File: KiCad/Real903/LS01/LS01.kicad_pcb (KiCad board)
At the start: 2 copper layers, 50.8 x 19 mm, 24 parts, among them J1 Conn_01x06, J2 Conn_01x03, J3 Conn_01x03

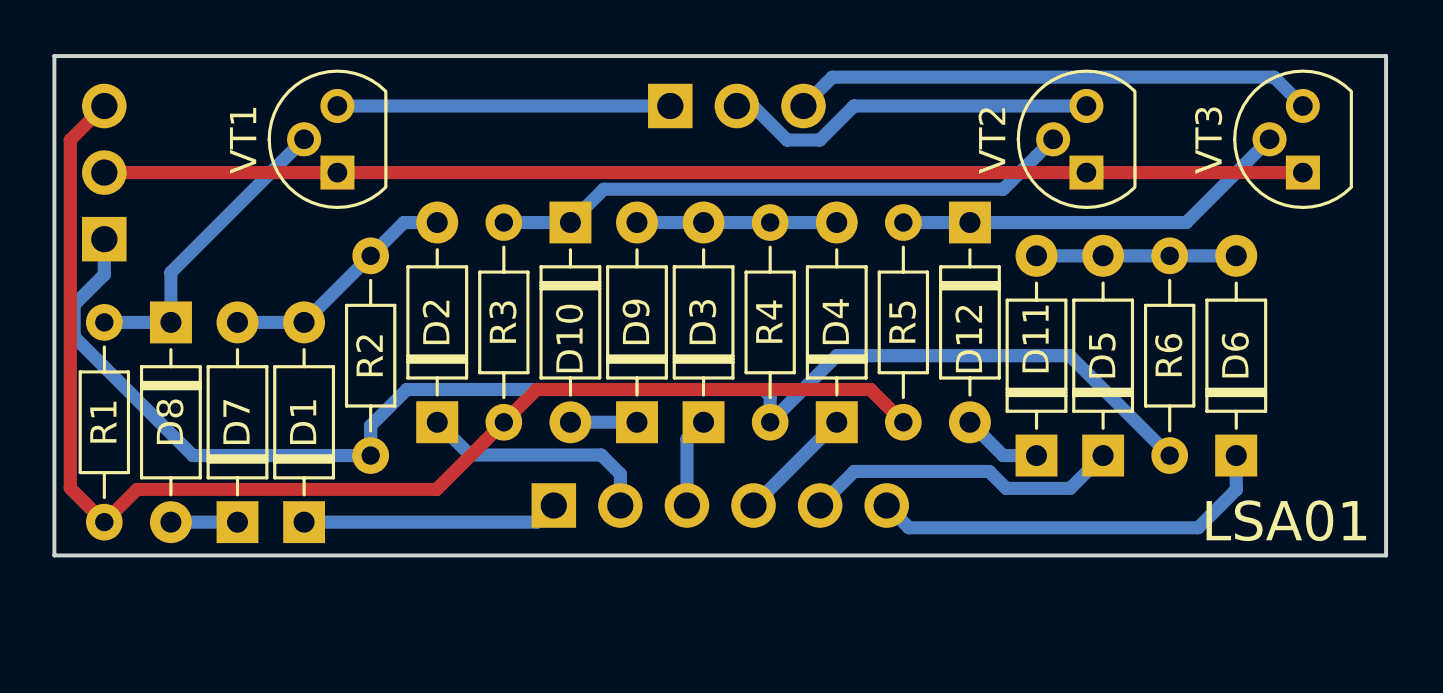
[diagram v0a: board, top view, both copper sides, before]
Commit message: New Kicad design files
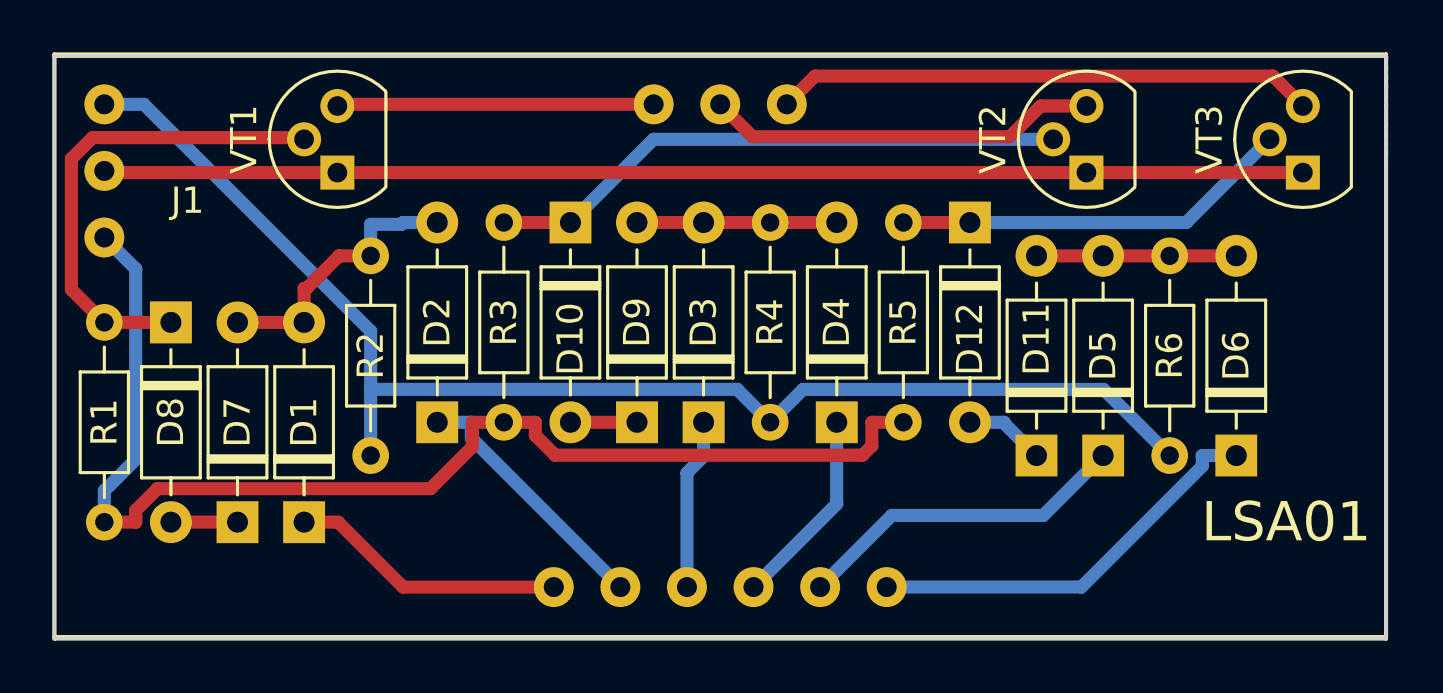
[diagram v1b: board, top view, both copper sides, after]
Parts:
- removed J2, J3: Conn_01x03, ELLIOTT:PinHeader_1x03_P2.54mm_Vertical
- J1: value Conn_01x06 -> LSAConnect; footprint ELLIOTT:PinHeader_1x06_P2.54mm_Vertical -> ELLIOTT:LSA; moved to F.Cu
- VT1, VT2, VT3: value BC -> BC547
- moved J1 18.5 mm to (100.3, 43.1), turned to 0 degrees
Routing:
- net Net-(D8-Pad1): track 12.1 -> 18.5 mm
- net -6v: track 50.0 -> 46.6 mm
- net 4: track 4.49 -> 7.60 mm
- net 3: track 3.44 -> 6.55 mm
- net +6v: track 53.3 -> 51.1 mm
- net Net-(D1-Pad2): track 9.20 -> 10.7 mm
- net 2: track 9.00 -> 9.94 mm
- net 1: track 9.79 -> 10.6 mm
- net 5: track 12.1 -> 12.9 mm
- net 13: track 20.0 -> 20.6 mm
- net 11: track 12.7 -> 12.1 mm
- net 12: track 14.4 -> 15.0 mm
- added copper zone on B.Cu, net 0v
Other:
- board size 50.8 x 19 mm -> 50.8 x 22.2 mm
